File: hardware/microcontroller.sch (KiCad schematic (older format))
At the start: 8 parts, among them J1 Conn_02x05_Odd_Even, U1 ESP-WROOM-32

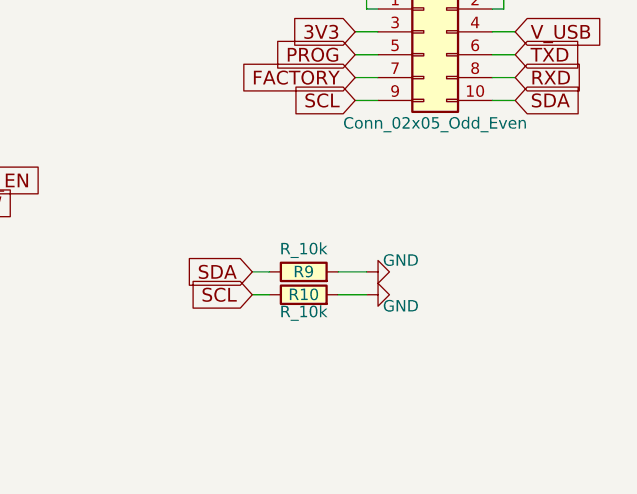
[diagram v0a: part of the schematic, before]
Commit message: update
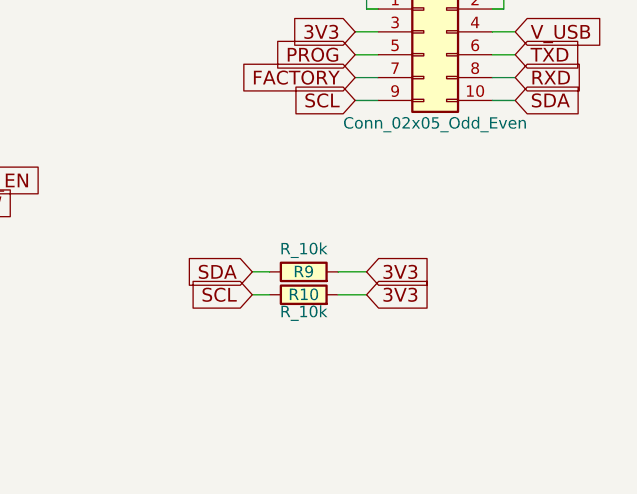
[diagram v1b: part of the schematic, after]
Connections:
- net 3V3: now also R10.2, R9.2
- net GND: no longer R10.2, R9.2
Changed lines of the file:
@@
-	0    -1   -1   0
-$EndComp
-$Comp
-L GND #PWR06
-U 1 1 59C84033
-P 8725 4300
-F 0 "#PWR06" H 8725 4050 50  0001 C CNN
-F 1 "GND" V 8675 4150 50  0000 C CNN
-F 2 "" H 8725 4300 50  0000 C CNN
-F 3 "" H 8725 4300 50  0000 C CNN
-	1    8725 4300
-	0    -1   -1   0
-$EndComp
-$Comp
-L GND #PWR07
-U 1 1 59C84056
-P 8725 4200
-F 0 "#PWR07" H 8725 3950 50  0001 C CNN
-F 1 "GND" V 8775 4050 50  0000 C CNN
-F 2 "" H 8725 4200 50  0000 C CNN
-F 3 "" H 8725 4200 50  0000 C CNN
-	1    8725 4200
 	0    -1   -1   0
 $EndComp
@@
 Wire Wire Line
 	8725 4300 8600 4300
+Text GLabel 8725 4200 2    60   Input ~ 0
+3V3
+Text GLabel 8725 4300 2    60   Input ~ 0
+3V3
 $EndSCHEMATC
